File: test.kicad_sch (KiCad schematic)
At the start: 43 parts, among them IC1 AS358AP-E1, J3 Transformer, Q1 2N4401, Q2 2N4401, Q3 2N4401, Q4 2N4403, Q5 TIP30C, Q6 2N4403, Q7 2N4401, Q8 2N4403, U1 TIP29C

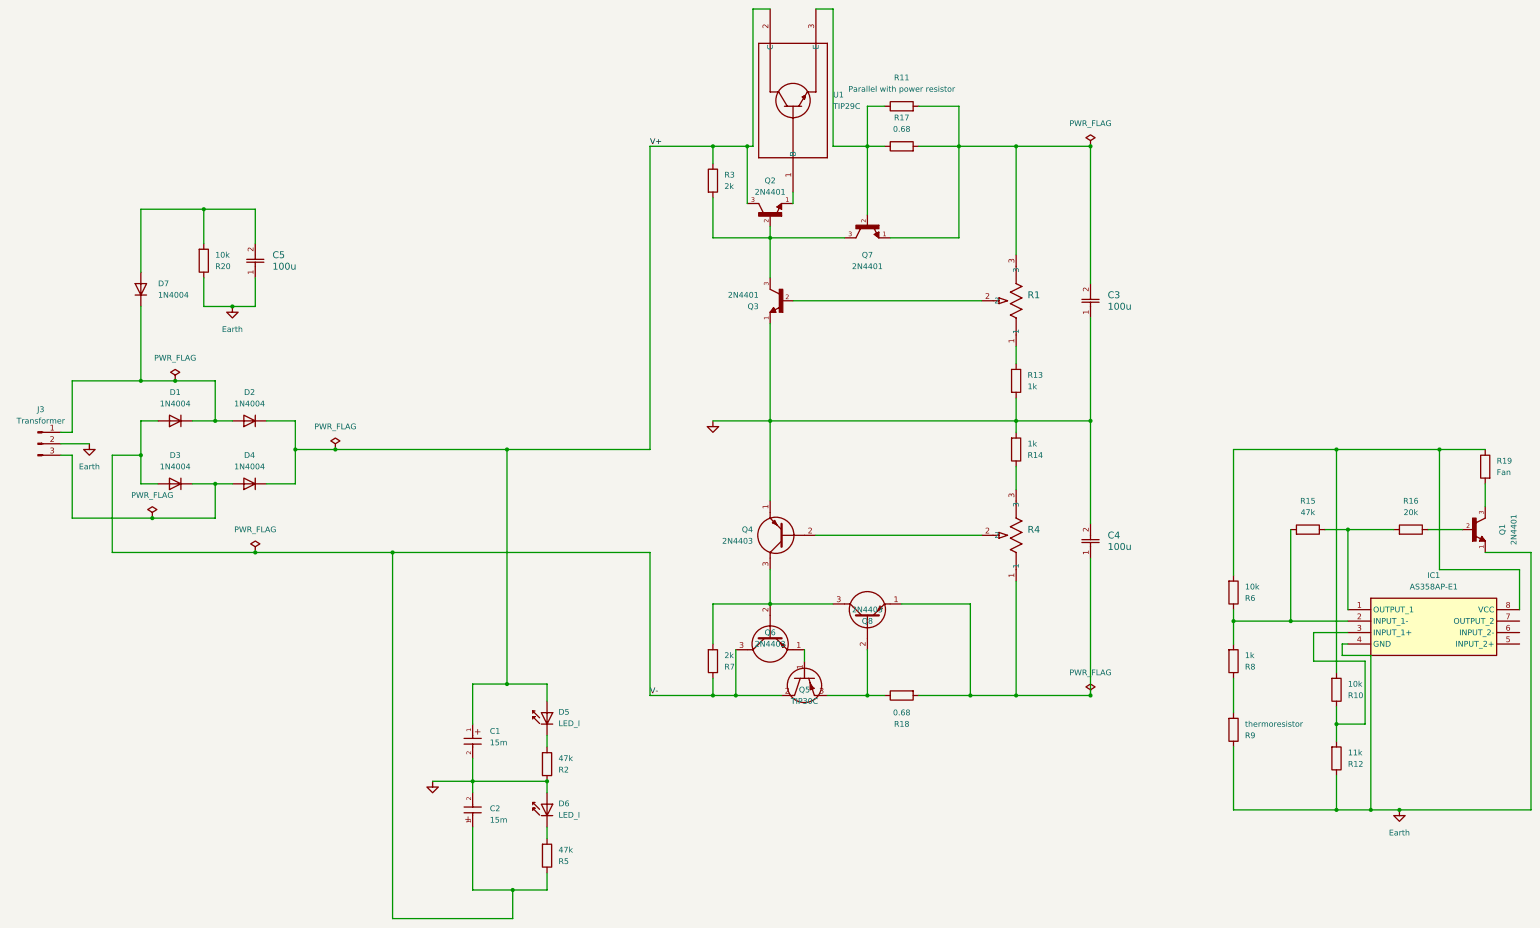
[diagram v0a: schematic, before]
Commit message: Updated by Bryce Thu 11/20/2025 22:02
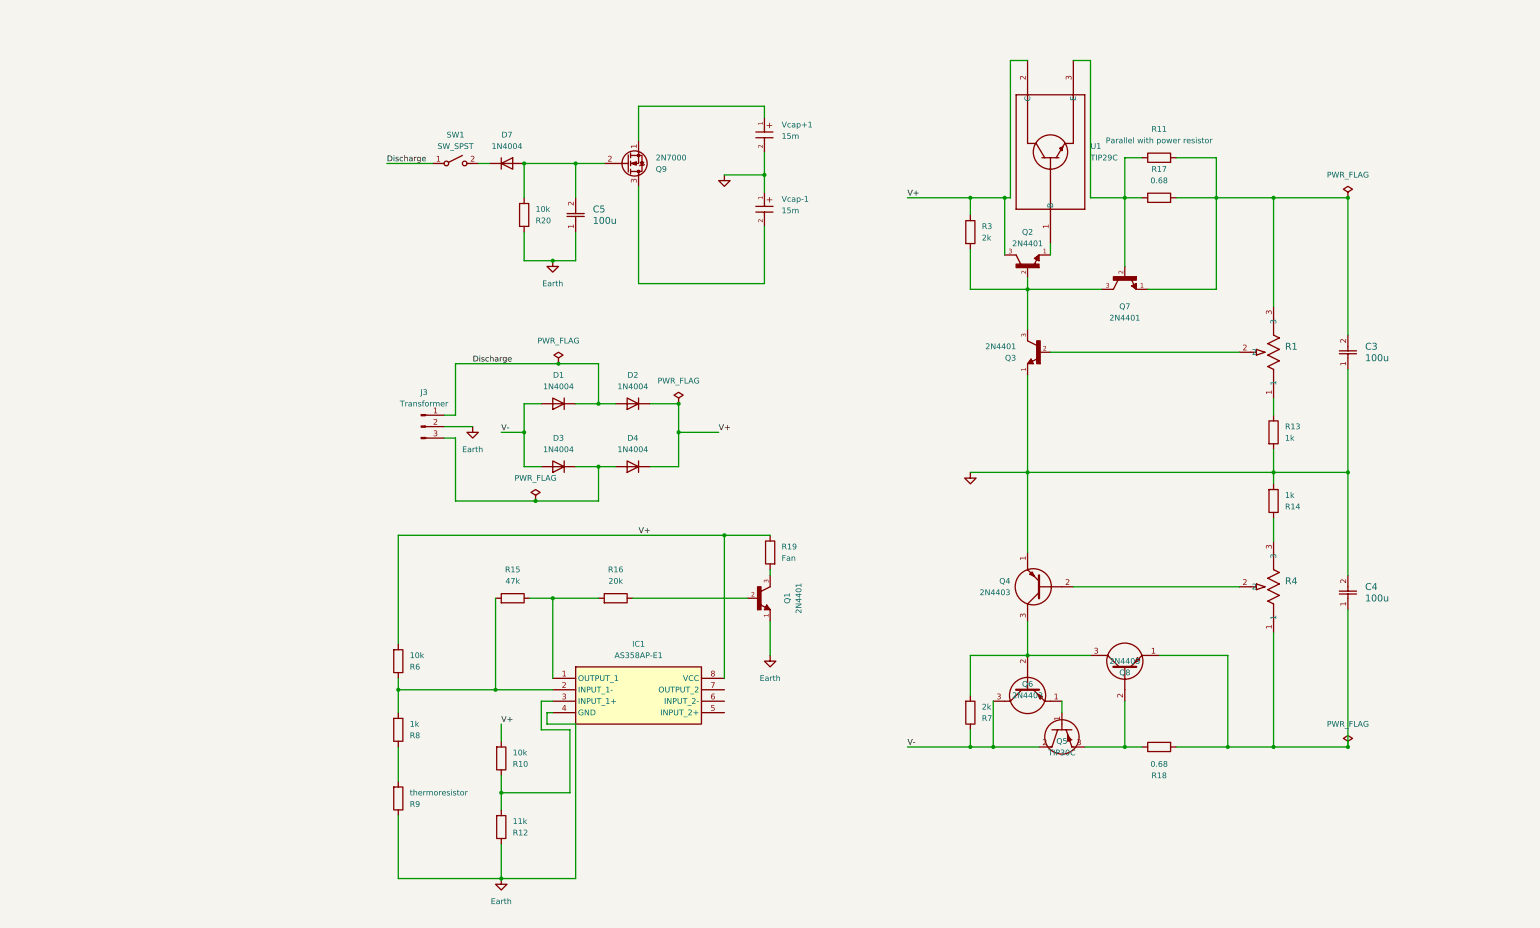
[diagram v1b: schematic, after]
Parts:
- removed D5, D6: LED_I, LED_THT:LED_D5.0mm, symbol LED:CQY99
- removed R2, R5: 47k, Resistor_THT:R_Axial_DIN0207_L6.3mm_D2.5mm_P15.24mm_Horizontal, symbol Device:R
- added Q9: 2N7000, Package_TO_SOT_THT:TO-92_Inline, symbol Transistor_FET:2N7000
- added SW1: SW_SPST, symbol Switch:SW_SPST
- IC1: footprint DIP762W56P254L930H431Q8N -> LIB_AS358AP-E1:DIP762W56P254L930H431Q8N
- R9: footprint Resistor_THT:R_Axial_DIN0207_L6.3mm_D2.5mm_P15.24mm_Horizontal -> Resistor_THT:R_Axial_DIN0204_L3.6mm_D1.6mm_P5.08mm_Horizontal
- renumbered C1 to Vcap+1, C2 to Vcap-1
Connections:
- net Earth: now also Vcap-1.1; no longer Vcap-1.2
- net V+: now also IC1.8 (VCC), R10.2, R19.1, R6.2; no longer Vcap+1.1
- net V-: no longer Vcap-1.1
- net Discharge: now reaches D1.1 (K), D2.2 (A), J3.1 (Pin_1)
- net Discharge: now also SW1.1 (A); no longer D7.1 (K)
- net at C5.2, D7.2 (A), R20.2: now also Q9.2 (G)
- new net: D7.1 (K), SW1.2 (B)
- new net: Q9.1 (S), Vcap+1.1
- new net: Q9.3 (D), Vcap-1.2
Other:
- moved on the sheet: C3, C4, C5, D1, D2, D3, D4, D7, IC1, J3, Q1, Q2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

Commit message: Updated by Bryce Thu 11/20/2025 22:43
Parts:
- SW1: footprint (none) -> Connector_Wire:SolderWire-0.1sqmm_1x02_P3.6mm_D0.4mm_OD1mm
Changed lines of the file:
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@@
 			)
 		)
-		(property "Footprint" ""
+		(property "Footprint" "Connector_Wire:SolderWire-0.1sqmm_1x02_P3.6mm_D0.4mm_OD1mm"
 			(at 35.56 29.21 0)
 			(effects
